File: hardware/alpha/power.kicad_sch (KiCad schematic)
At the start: 1 part, among them U2 TPS61170DRVR

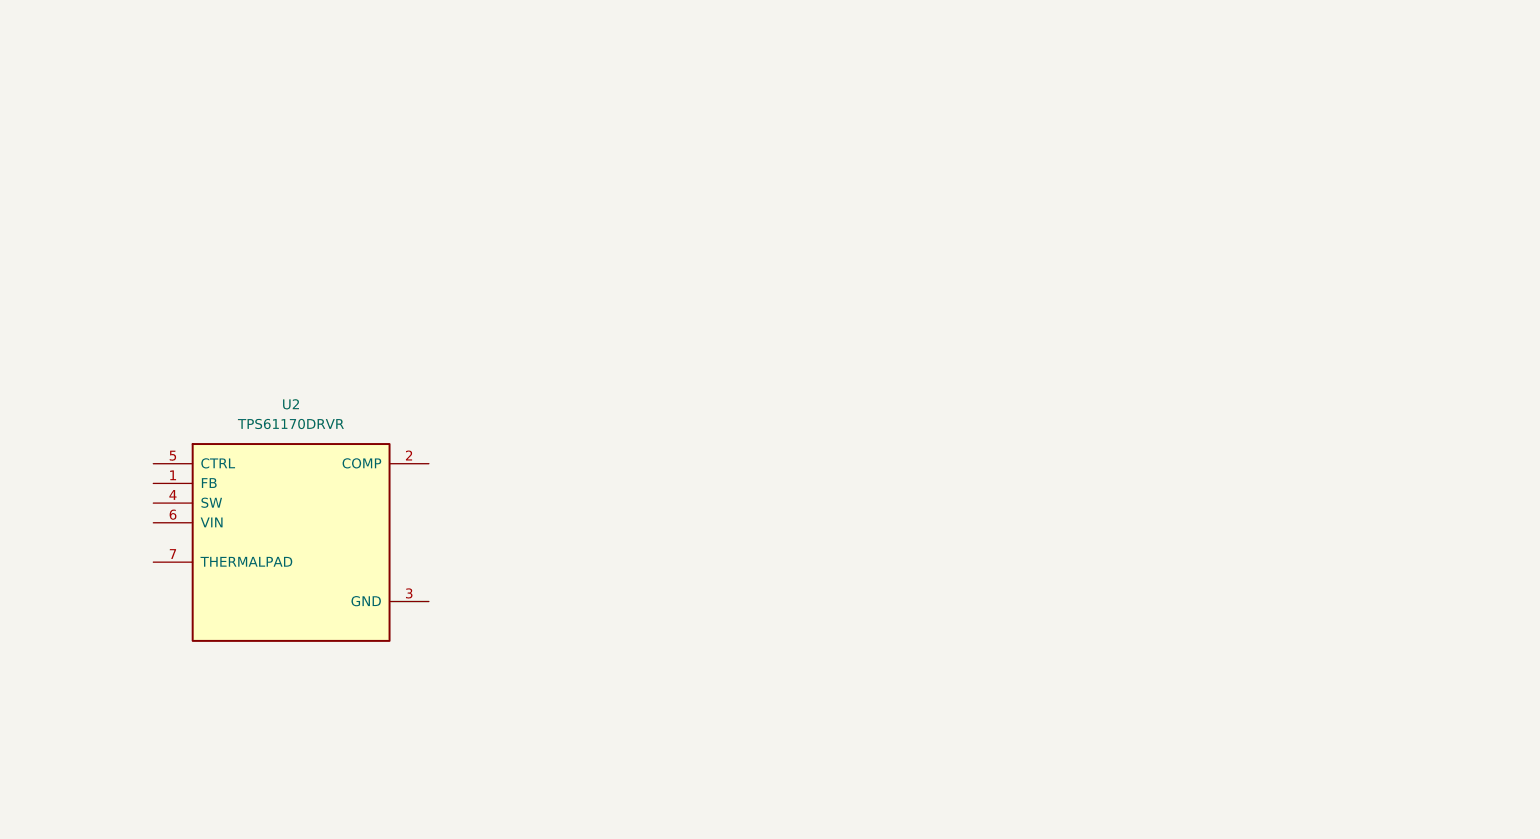
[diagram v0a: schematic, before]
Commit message: Updated
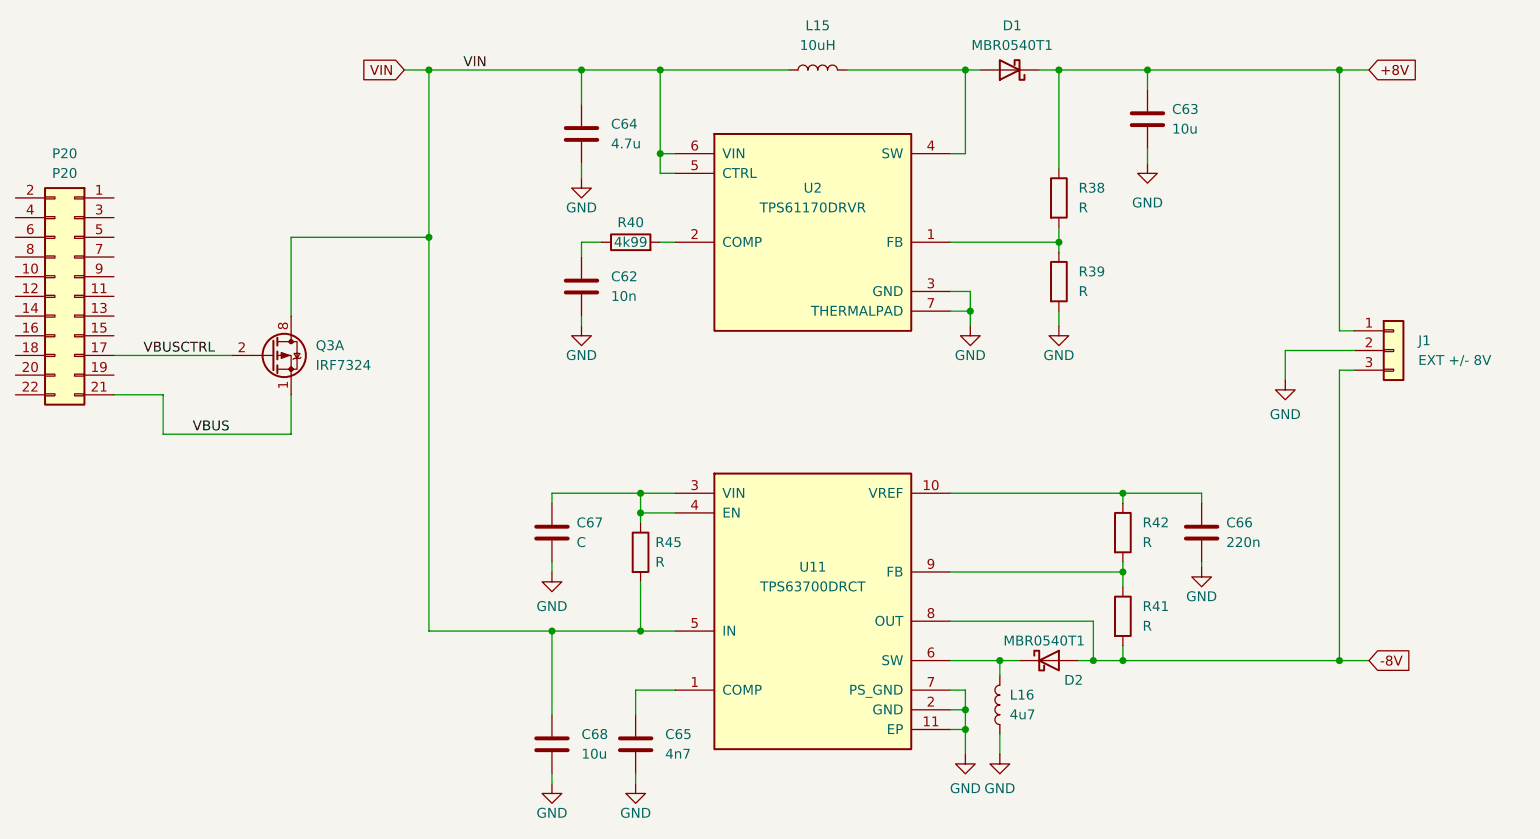
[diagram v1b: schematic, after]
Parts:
- added C62: 10n, symbol Device:C
- added C63, C68: 10u, symbol Device:C
- added C64: 4.7u, symbol Device:C
- added C65: 4n7, symbol Device:C
- added C66: 220n, symbol Device:C
- added C67: C, symbol Device:C
- added D1, D2: MBR0540T1, symbol Device:D_Schottky
- added J1: EXT +/- 8V, symbol Connector_Generic:Conn_01x03
- added L15: 10uH, symbol Device:L
- added L16: 4u7, symbol Device:L
- added P20: P20, symbol Connector_Generic:Conn_02x11_Odd_Even
- added Q3: IRF7324, Package_SO:SOIC-8_3.9x4.9mm_P1.27mm, symbol Transistor_FET:IRF7324
- added R38, R39, R41, R42, R45: R, symbol Device:R
- added R40: 4k99, symbol Device:R
- added U11: TPS63700DRCT, TPS63700DRCT:VREG_V62_16624-01YE, symbol TPS63700:TPS63700DRCT
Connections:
- net at U2.1 (FB): now also R38.2, R39.1
- net at U2.2 (COMP): now also R40.2
- net GND: now reaches U2.3 (GND)
- net GND: now also U2.7 (THERMALPAD), C62.2, C63.2, C64.2, C65.2, C66.2, C67.2, C68.2, J1.2 (Pin_2), L16.1, R39.2, U11.11 (EP), U11.2 (GND), U11.7 (PS_GND)
- net at U2.4 (SW): now also D1.2 (A), L15.2
- net VIN: now reaches U2.5 (CTRL)
- net VIN: now also U2.6 (VIN), C64.1, C68.1, L15.1, Q3.7 (D1), Q3.8 (D1), R45.2, U11.5 (IN)
- new net: C67.1, R45.1, U11.3 (VIN), U11.4 (EN)
- new net: C65.1, U11.1 (COMP)
- new net: R41.1, R42.2, U11.9 (FB)
- new net: D2.1 (K), L16.2, U11.6 (SW)
- new net: C62.1, R40.1
- new net: C66.1, R42.1, U11.10 (VREF)
- new net +8V: C63.1, D1.1 (K), J1.1 (Pin_1), R38.1
- new net -8V: D2.2 (A), J1.3 (Pin_3), R41.2, U11.8 (OUT)
- new net VBUS: P20.21 (Pin_21), Q3.1 (S1)
- new net VBUSCTRL: P20.17 (Pin_17), Q3.2 (G1)
